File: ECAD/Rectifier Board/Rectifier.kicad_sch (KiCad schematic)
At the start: 36 parts, among them J1 MAINS, Q1 IXFH48N60X3, U2 IR1153S

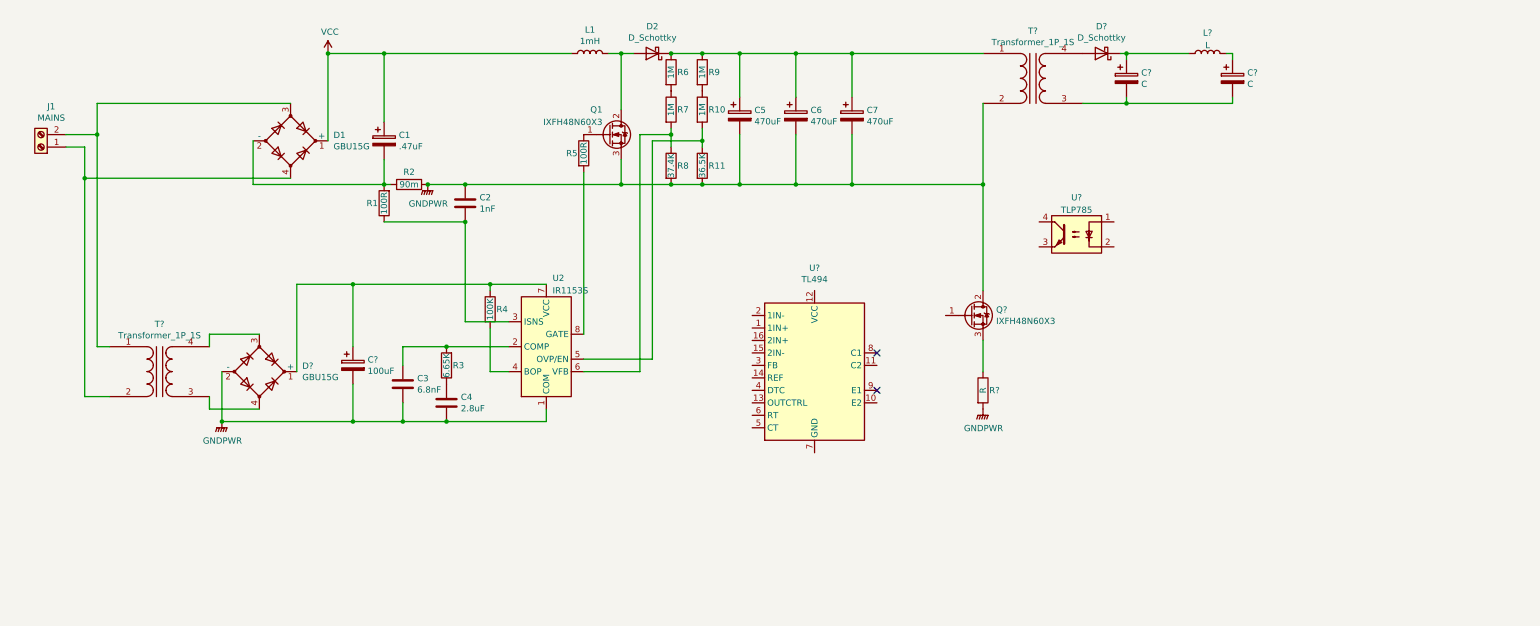
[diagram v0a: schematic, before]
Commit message: Place all components, divide sch
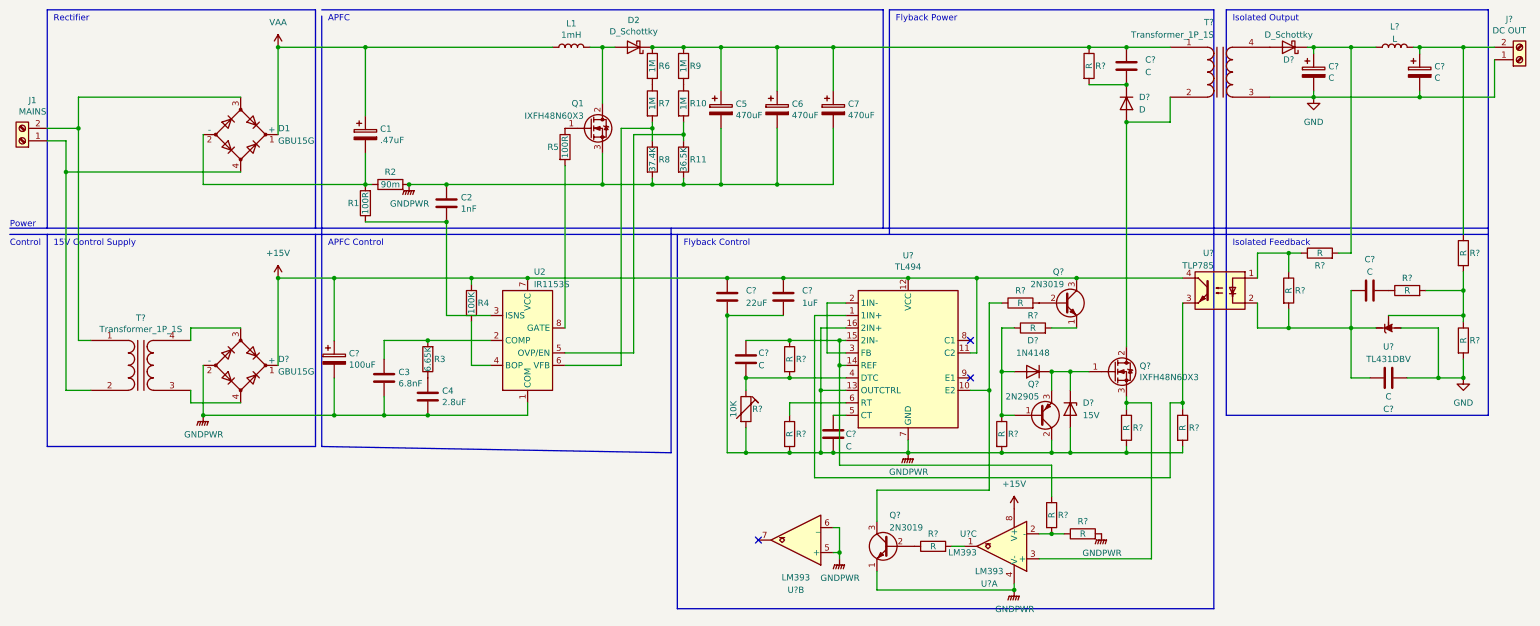
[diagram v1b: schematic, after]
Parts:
- removed R?: R, symbol Device:R
- added C? (x5): C, symbol Device:C
- added C?: 1uF, symbol Device:C
- added C?: 22uF, symbol Device:C
- added D?: D, symbol Device:D
- added D?: 1N4148, symbol Device:D
- added D?: 15V, symbol Device:D_Zener
- added J?: DC OUT, symbol Connector:Screw_Terminal_01x02
- added Q? (x2): 2N3019, symbol Device:Q_NPN_EBC
- added Q?: 2N2905, symbol Device:Q_PNP_BCE
- added R? (x16): R, symbol Device:R
- added R?: 10K, symbol Device:R_Trim
- added U? (x3): LM393, symbol Comparator:LM393
- added U?: TL431DBV, Package_TO_SOT_SMD:SOT-23-5, symbol Reference_Voltage:TL431DBV
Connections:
- net GNDPWR: now also U?.13 (OUTCTRL), U?.16 (2IN+), U?.7 (GND), C?.2, C?.2, C?.2, D?.2 (A), Q?.1 (E), Q?.2 (C), R?.2, R?.2, R?.2, R?.2, R?.2, R?.2, U?.4 (V-), U?.5 (+), U?.6 (_); no longer Q?.2 (D), T?.2 (AB)
- net +15V: now reaches C?.1, D?.1 (+), R4.1, U2.7 (VCC)
- net +15V: now also U?.11 (C2), U?.12 (VCC), U?.4, C?.1, C?.1, Q?.3 (C), U?.8 (V+)
- net at C5.1, C6.1, C7.1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: now also C?.1, R?.1
- net at U?.1 (1IN+): now also U?.3, R?.1
- net at U?.10 (E2): now also Q?.3 (C), R?.1
- net at U?.14 (REF): now also U?.15 (2IN-), C?.1, R?.1, R?.1
- net at U?.2 (1IN-): now also U?.3 (FB)
- net at U?.4 (DTC): now also C?.2, R?.1, R?.2
- net at U?.5 (CT): now also C?.1
- net at U?.6 (RT): now also R?.1
- net GND: now reaches C?.2, C?.2, T?.3 (SA)
- net GND: now also C?.2, J?.1 (Pin_1), R?.2, U?.5 (A)
- net at Q?.1 (G): now also D?.1 (K), D?.1 (K), Q?.3 (E)
- net at Q?.3 (S): now also R?.1, U?.3 (+)
- net at C?.1, D?.1 (K), L?.1: now also R?.2
- net at C?.1, L?.2: now also J?.2 (Pin_2), R?.1
- net at U?.1: now also R?.1, R?.1
- net at U?.2: now also C?.1, C?.1, R?.2, U?.3 (K)
- net VCC renamed VAA
- new net: C?.2, D?.1 (K), R?.2
- new net: D?.2 (A), Q?.2 (D), T?.2 (AB)
- new net: D?.2 (A), Q?.1 (B), R?.1, R?.1
- new net: R?.1, R?.2, U?.2 (-)
- new net: Q?.1 (E), R?.2
- new net: Q?.2 (B), R?.2
- new net: Q?.2 (B), R?.1
- new net: R?.2, U?.1
- new net: R?.1, R?.2, R?.2, U?.4 (REF)
- new net: C?.2, R?.1
- no-connect marks 2 -> 3
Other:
- note added: "15V Control Supply"
- note added: "APFC"
- note added: "APFC Control"
- note added: "Control"
- note added: "Flyback Control"
- note added: "Flyback Power"
- note added: "Isolated Feedback"
- note added: "Isolated Output"
- note added: "Power"
- note added: "Rectifier"
- moved on the sheet: C1, C2, C3, C4, C5, C6, C7, C?, D1, D2, D?, J1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
